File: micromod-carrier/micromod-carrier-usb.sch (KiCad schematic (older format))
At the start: 60 parts, among them J2 USB_C_Receptacle_USB2.0, J8 USBHUB, J9 USBHOST, U1 GL850, U2 FT4232H-56Q-REEL, U3 74HC595, X1 12MHz, X2 12MHz

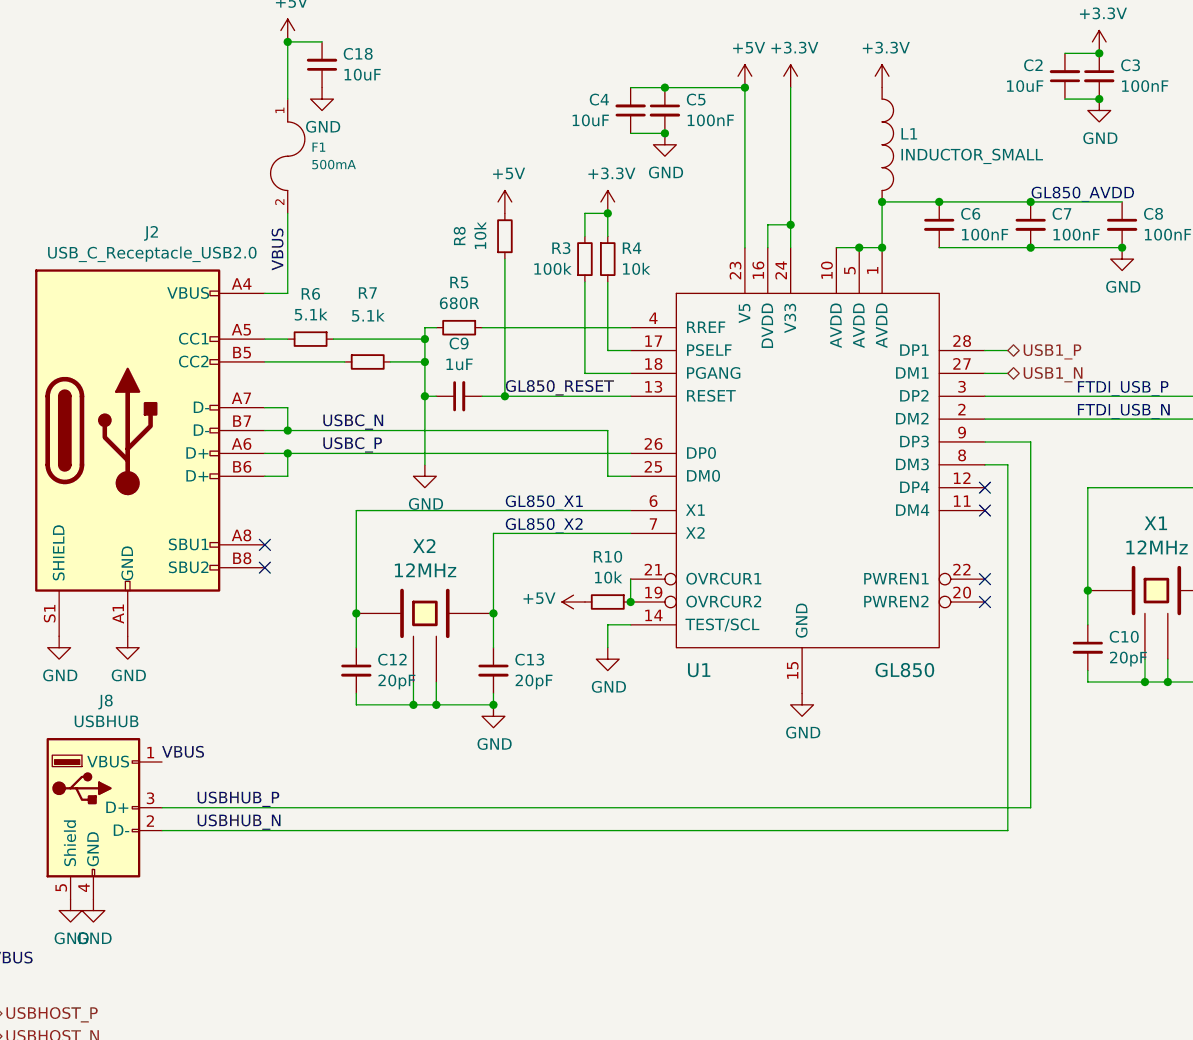
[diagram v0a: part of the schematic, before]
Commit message: micromod-carrier: progress commit
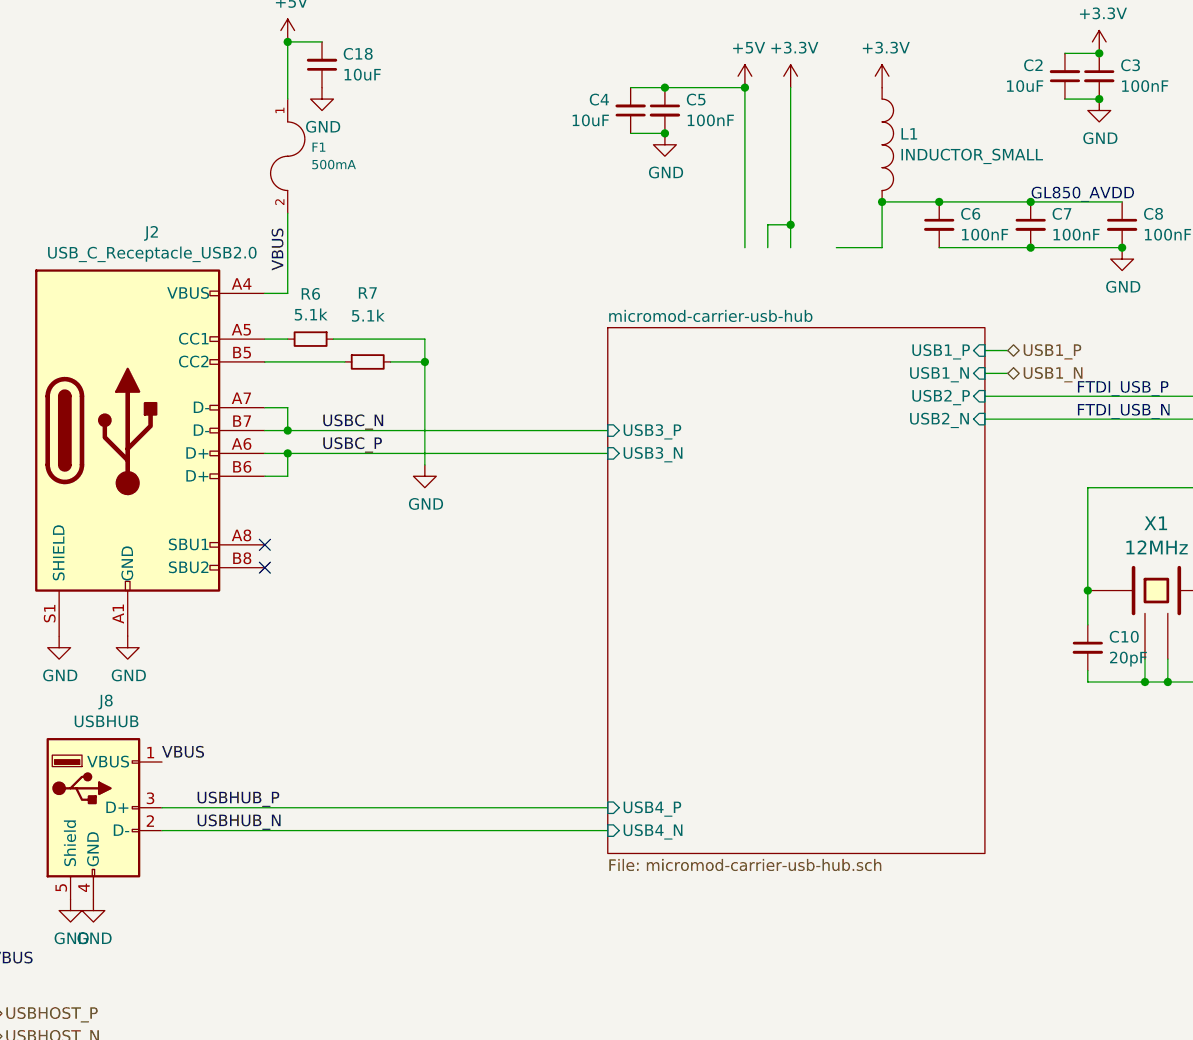
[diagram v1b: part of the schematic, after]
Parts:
- removed C12, C13: 20pF, tom-passives:C_0603_1608Metric, symbol jlcpcb-basic-mlcc-0603:20pF
- removed C9: 1uF, tom-passives:C_0603_1608Metric, symbol jlcpcb-basic-mlcc-0603:1uF
- removed R10, R4, R8: 10k, tom-passives:R_0603_1608Metric, symbol jlcpcb-basic-resistor-0603:10k
- removed R3: 100k, tom-passives:R_0603_1608Metric, symbol jlcpcb-basic-resistor-0603:100k
- removed R5: 680R, tom-passives:R_0603_1608Metric, symbol jlcpcb-basic-resistor-0603:680R
- removed U1: GL850, tom-semiconductors:SSOP-28_5.3x10.2mm_P0.65mm, symbol tom-semiconductors:GL850
- removed X2: 12MHz, tom-passives:Crystal_SMD_3225-4Pin_3.2x2.5mm, symbol tom-passives:CRYSTAL_4PIN
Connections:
- net micromod-carrier-usb-hub/USB2_N: now reaches U2.7 (DM)
- net micromod-carrier-usb-hub/USB2_P: now reaches U2.8 (DP)
- no-connect marks 30 -> 26
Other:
- note removed: "GL850_X1"
- note removed: "GL850_X2"
